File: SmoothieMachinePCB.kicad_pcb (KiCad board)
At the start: 2 copper layers, 50 parts, among them J1 Up Button, J10 Vin, J11 LCD I2C Adapter, J2 Down Button, J3 Next Ingredient Button, J4 Next Recipe Button, J5 Solenoid Valve, J6 Stepper Motor 2, J8 Stepper Motor 1, J9 LoadCell, U1 ESP32-S3-WROOM-2, U2 FSA2567MPX, U3 DRV8825PWP, U4 VN10KN3-G, U6 NAU7802SGI, U7 XL1509-3.3

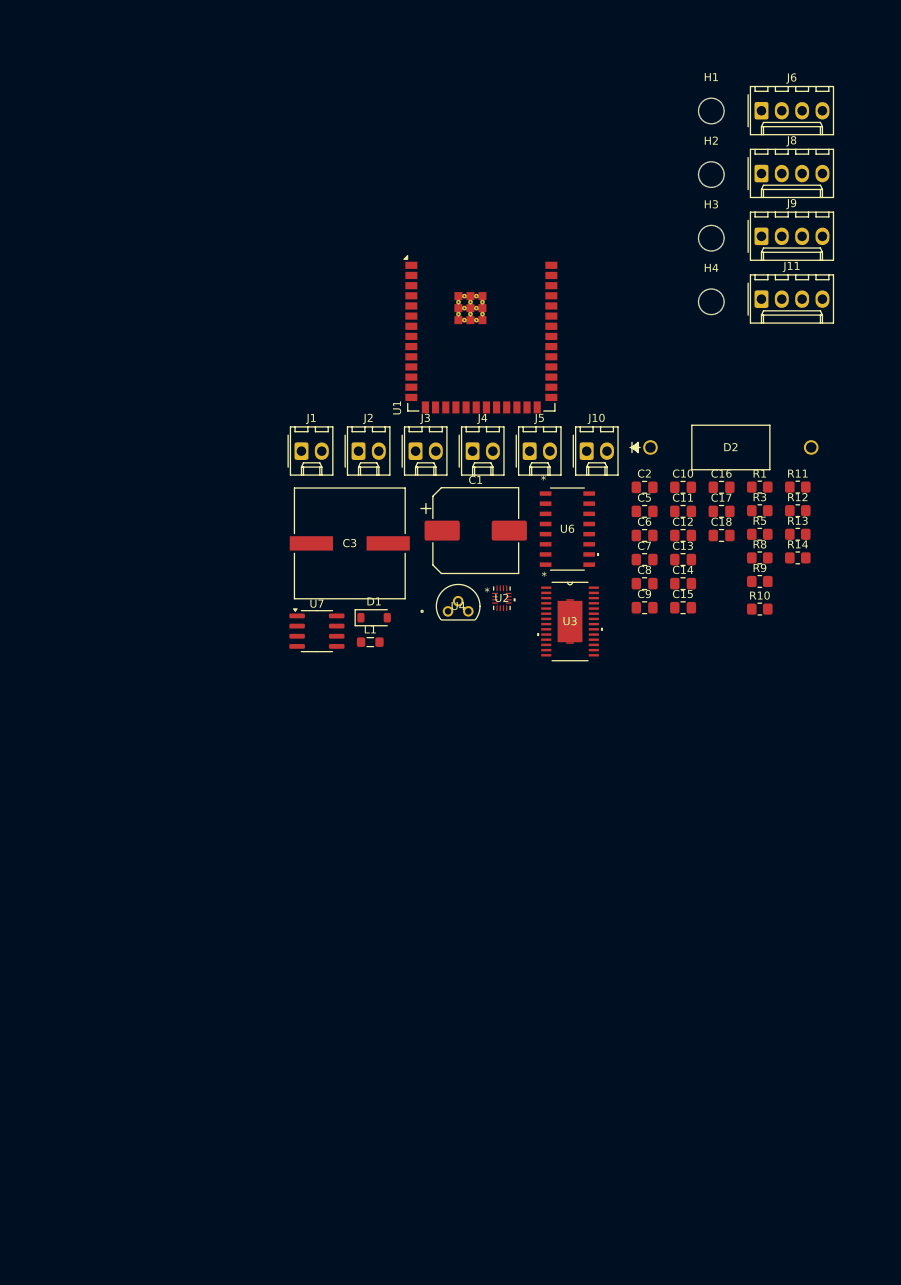
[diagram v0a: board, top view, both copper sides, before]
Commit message: Second round pcb files
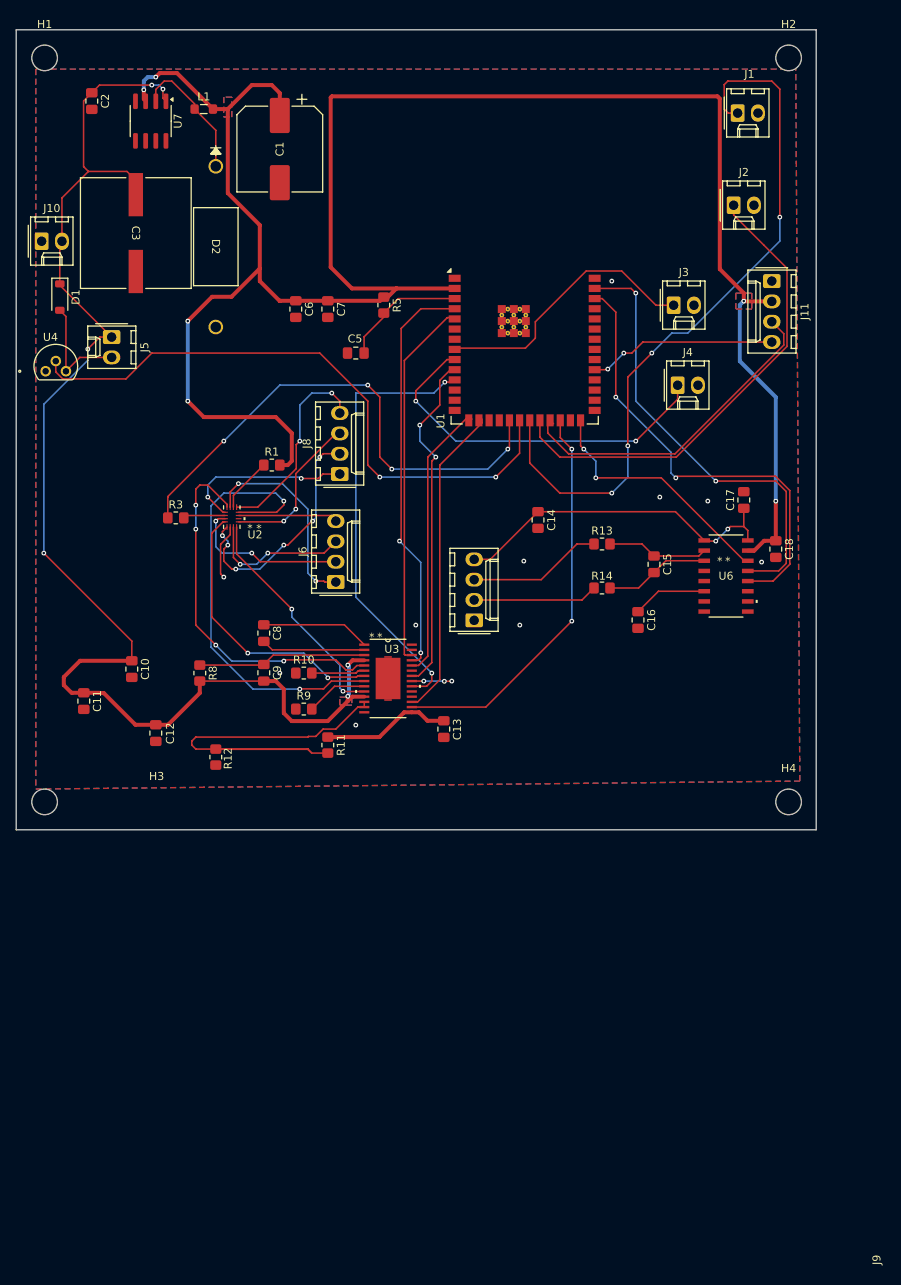
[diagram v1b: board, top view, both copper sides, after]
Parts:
- moved H3 109.1 mm to (88.6, 144.1)
- moved C2 84.3 mm to (94.5, 56.5), turned to -90 degrees
- moved H1 83.6 mm to (88.6, 51.1)
- moved J6 79.4 mm to (125.0, 116.6), turned to 90 degrees
- moved R12 79.0 mm to (110.0, 138.5), turned to -90 degrees
- moved C11 78.6 mm to (93.5, 131.5), turned to -90 degrees
- moved J10 73.0 mm to (88.2, 74.0)
- moved R3 73.0 mm to (105.0, 108.6)
- moved C10 72.6 mm to (99.5, 127.5), turned to -90 degrees
- moved R8 71.5 mm to (108.0, 128.0), turned to -90 degrees
- moved C12 70.4 mm to (102.5, 135.5), turned to -90 degrees
- moved L1 69.8 mm to (108.5, 57.5)
- moved J1 69.0 mm to (175.2, 58.0)
- moved U7 67.1 mm to (101.9, 59.0), turned to -90 degrees
- moved R11 67.0 mm to (124.0, 137.0), turned to -90 degrees
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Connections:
- D2 pad 1: /VDD33 -> Net-(D2-K)
- J11 pad 2: /VDD5 -> /VDD33
- L1 pad 1: /VDD33 -> Net-(D2-K)
- R3 pad 1: /MotorSelect -> /MOTORSELECT
- U7 pad 2: /VDD33 -> Net-(D2-K)
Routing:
- net /VDD33: track 0.00 -> 262.7 mm, vias 0 -> 6
- net +12V: track 0.00 -> 169.3 mm, vias 0 -> 6
- net /UP_BUTTON: track 0.00 -> 90.0 mm, vias 0 -> 4
- net /SOLENOID_VALVE: track 0.00 -> 77.5 mm, vias 0 -> 2
- net /MOTORSELECT: track 0.00 -> 64.4 mm, vias 0 -> 4
- net /DOWN_BUTTON: track 0.00 -> 60.2 mm
- net /DRDY: track 0.00 -> 57.6 mm, vias 0 -> 2
- net /SCLK: track 0.00 -> 56.5 mm, vias 0 -> 2
- net /BOUT2C: track 0.00 -> 56.1 mm, vias 0 -> 2
- net /DIR: track 0.00 -> 55.7 mm, vias 0 -> 2
- net /MODE1: track 0.00 -> 51.3 mm, vias 0 -> 2
- net /NRESET: track 0.00 -> 50.1 mm, vias 0 -> 2
- net /MODE2: track 0.00 -> 46.6 mm
- net /NEXT_RECEP_BUTTON: track 0.00 -> 46.5 mm, vias 0 -> 2
- net /AOUT1C: track 0.00 -> 46.2 mm, vias 0 -> 4
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- added copper zone on B.Cu, net +12V
- added copper zone on F.Cu, net +12V
- added copper zone on B.Cu, net /VDD33
- added copper zone on F.Cu, net /VDD33
- added copper zone on B.Cu, net GND
- added copper zone on F.Cu, net GND
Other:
- board outline added: 100 x 100 mm
